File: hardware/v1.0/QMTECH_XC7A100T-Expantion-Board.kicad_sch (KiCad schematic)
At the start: 18 parts, among them J1 Micro_SD_Card_Det1, J2 Conn_01x34, J3 USB_C_Receptacle_USB2.0_16P, J4 Conn_01x34, U3 TPS25200

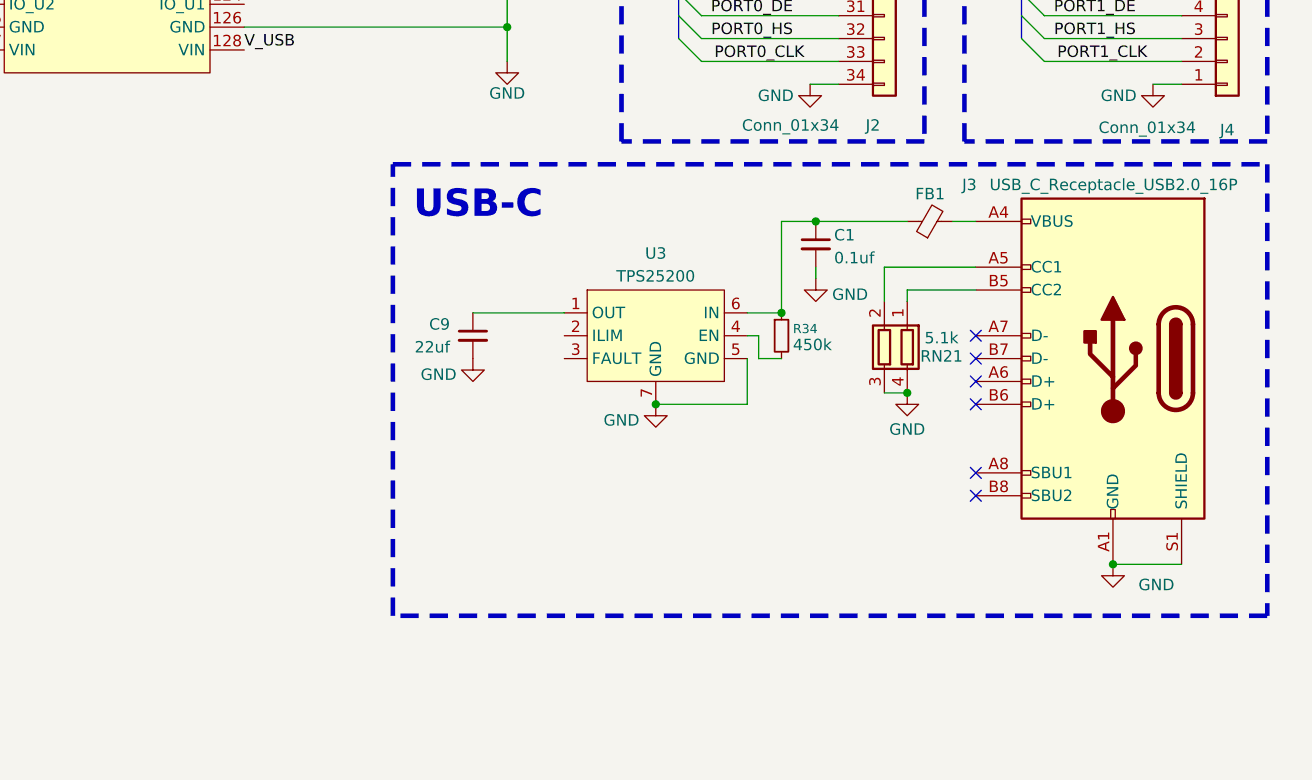
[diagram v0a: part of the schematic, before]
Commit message: changes
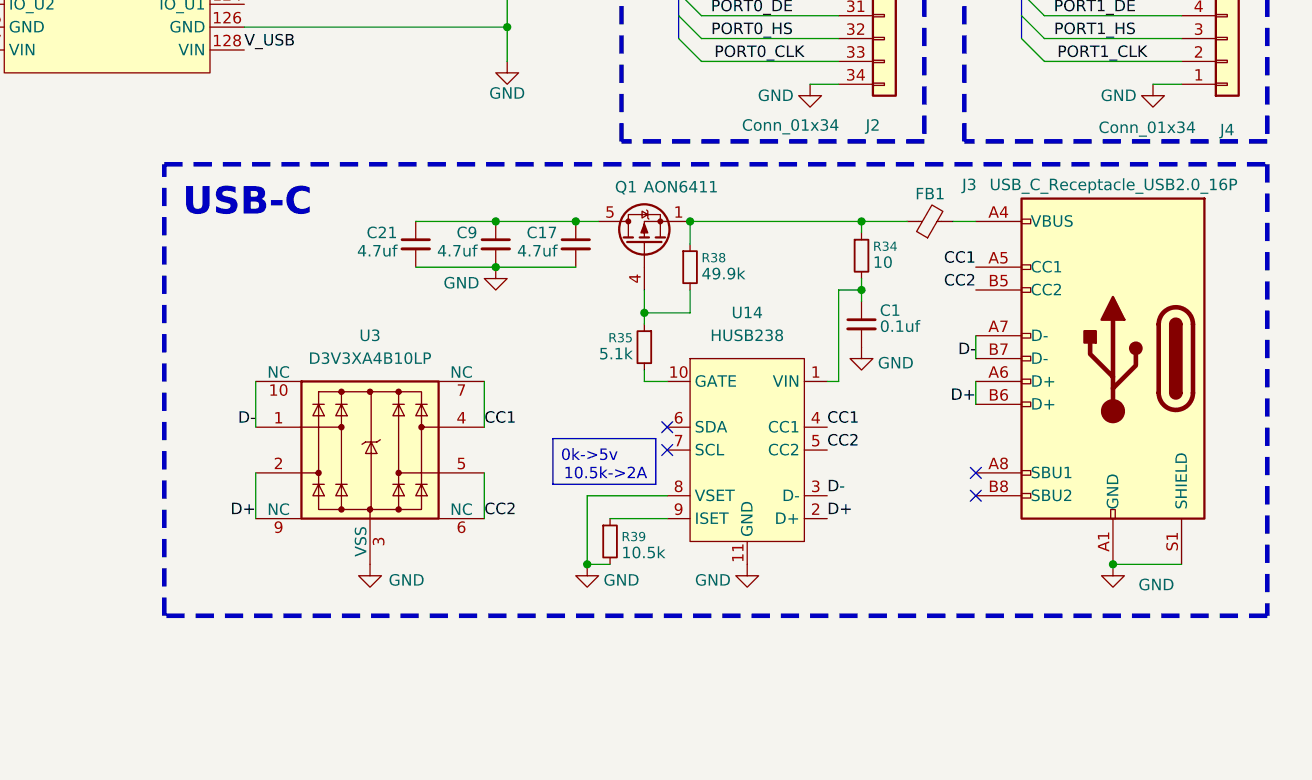
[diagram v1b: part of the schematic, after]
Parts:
- removed RN21: 5.1k, symbol Device:R_Pack02
- removed U3: TPS25200, Package_SON:WSON-6-1EP_2x2mm_P0.65mm_EP1x1.6mm, symbol mylib:TPS25200
- added C17, C21: 4.7uf, symbol Device:C_Small
- added Q1: AON6411, Package_DFN_QFN:AO_DFN-8-1EP_5.55x5.2mm_P1.27mm_EP4.12x4.6mm, symbol Transistor_FET:AON6411
- added R35: 5.1k, symbol Device:R_Small
- added R38: 49.9k, symbol Device:R_Small
- added R39: 10.5k, symbol Device:R_Small
- added U14: HUSB238, Package_DFN_QFN:DFN-10-1EP_3x3mm_P0.5mm_EP1.65x2.38mm_ThermalVias, symbol mylib:HUSB238
- added U3: D3V3XA4B10LP, Package_DFN_QFN:Diodes_UDFN-10_1.0x2.5mm_P0.5mm, symbol Power_Protection:D3V3XA4B10LP
- C9: value 22uf -> 4.7uf
- R34: value 450k -> 10
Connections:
- net GND: now also C17.2, C21.2, R39.2, U14.11 (GND), U14.8 (VSET), U3.3 (VSS), U3.8 (VSS)
- net at C9.1: now also C17.1, C21.1, Q1.5 (D)
- net at R34.2: now also C1.1, U14.1 (VIN)
- net at FB1.1, R34.1: now also Q1.1 (S), Q1.2 (S), Q1.3 (S), R38.1; no longer C1.1
- net CC2: now reaches J3.B5 (CC2)
- net CC2: now also U14.5 (CC2), U3.5, U3.6 (NC)
- net CC1: now reaches J3.A5 (CC1)
- net CC1: now also U14.4 (CC1), U3.4, U3.7 (NC)
- net D+: now reaches J3.A6 (D+)
- net D+: now also J3.B6 (D+), U14.2 (D+), U3.2, U3.9 (NC)
- net D-: now reaches J3.A7 (D-)
- net D-: now also J3.B7 (D-), U14.3 (D-), U3.1, U3.10 (NC)
- new net: R39.1, U14.9 (ISET)
- new net: Q1.4 (G), R35.1, R38.2
- new net: R35.2, U14.10 (GATE)
- no-connect marks 6 -> 4
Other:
- note added: "0k->5v"
- note added: "10.5k->2A"
- moved on the sheet: C1, C9
